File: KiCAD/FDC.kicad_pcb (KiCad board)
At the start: 2 copper layers, 72.6 x 65.5 mm, 26 parts, among them J2 Conn_02x20_Odd_Even, J3 SD_Card, Q1 SSM3K324RLFCT-ND, Q2 SSM3K324RLFCT-ND, U1 SN74LVCC4245ADWR, U2 Pico, U3 SN74LVCC4245ADWR, U4 SN74LVCC4245ADWR, U5 SN74LVCC4245ADWR

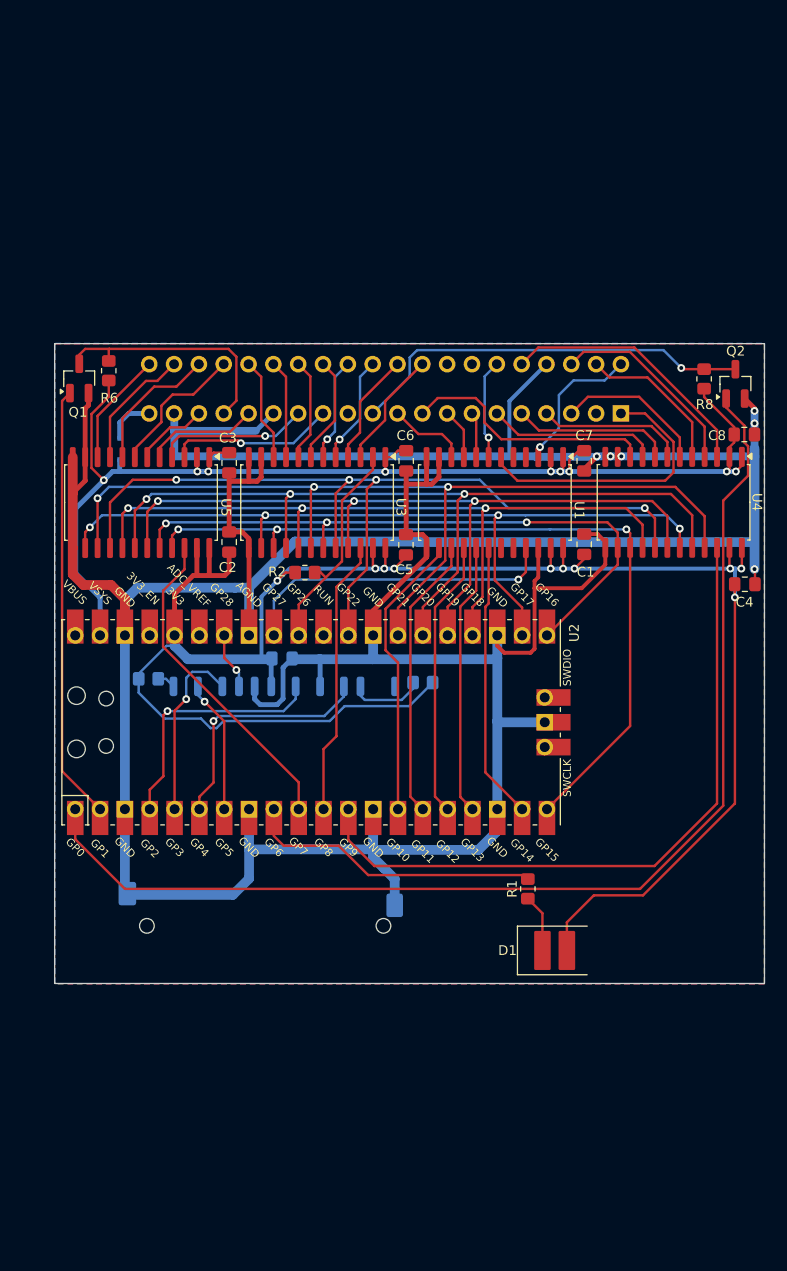
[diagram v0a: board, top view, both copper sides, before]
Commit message: First upload of test board.
First upload of test board.
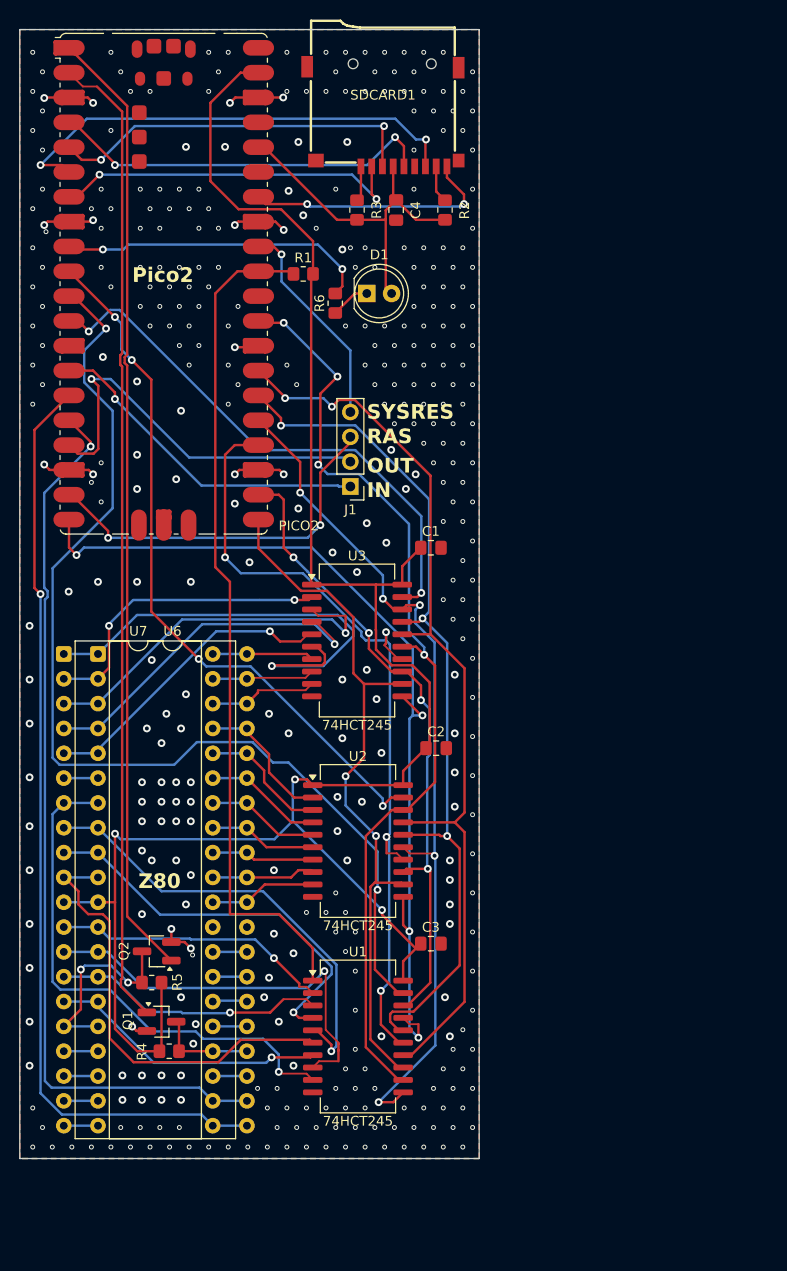
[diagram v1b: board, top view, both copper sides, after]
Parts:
- removed the C4 at (182.7, 80.7)
- removed C5, C6, C7, C8: 100nF, Capacitor_SMD:C_0805_2012Metric_Pad1.18x1.45mm_HandSolder
- removed D2: PMEG4010CEJ, Diode_SMD:D_SOD-323F
- removed J2: Conn_02x20_Odd_Even, Connector_PinSocket_2.54mm:PinSocket_2x20_P2.54mm_Vertical
- removed J3: SD_Card, Connector_Card:SD_Kyocera_145638009511859+
- removed the R2 at (137.7, 79.6)
- removed U4, U5: SN74LVCC4245ADWR, Package_SO:SOIC-24W_7.5x15.4mm_P1.27mm
- added J1: Conn_01x04, Connector_PinHeader_2.54mm:PinHeader_1x04_P2.54mm_Vertical, F.Cu at (142.3, 70.7)
- added R1: 1k, Resistor_SMD:R_0805_2012Metric_Pad1.20x1.40mm_HandSolder, F.Cu at (137.5, 49.0)
- added SDCARD1: ST-TF-003A, 00-ProjectLib:MicroSD_Card_TB, F.Cu at (145.7, 38.8)
- added U2: 74HCT245, Package_SO:SOIC-20W_7.5x15.4mm_P1.27mm, F.Cu at (143.1, 107.0)
- added U6: Z80, Package_DIP:DIP-40_W15.24mm, F.Cu at (116.5, 87.9)
- added U7: Z80, Package_DIP:DIP-40_W15.24mm, F.Cu at (113.0, 87.9)
- C4: renamed from C9; moved to F.Cu
- D1: footprint LED_SMD:LED_2816_7142Metric_Pad3.20x4.45mm_HandSolder -> LED_THT:LED_D5.0mm
- PICO2: renamed from U2; value Pico -> Pico 2; footprint MCU_RaspberryPi_and_Boards:RPi_Pico_SMD_TH -> Module:RaspberryPi_Pico_SMD
- Q1, Q2: value SSM3K324RLFCT-ND -> 2N7002
- R2: renamed from R3; moved to F.Cu
- R3: renamed from R4; moved to F.Cu
- U1, U3: value SN74LVCC4245ADWR -> 74HCT245; footprint Package_SO:SOIC-24W_7.5x15.4mm_P1.27mm -> Package_SO:SOIC-20W_7.5x15.4mm_P1.27mm
- moved R5 83.7 mm to (122.0, 121.5), turned to 0 degrees
- moved Q2 82.9 mm to (122.5, 118.3), turned to 180 degrees
- moved D1 69.9 mm to (144.0, 51.0)
- moved R4 69.9 mm to (123.8, 128.5), turned to 180 degrees
- moved Q1 66.3 mm to (123.0, 125.5), turned to 0 degrees
- moved R6 63.1 mm to (140.8, 52.0)
- moved U1 56.4 mm to (143.1, 127.0), turned to 0 degrees
- moved C3 53.3 mm to (150.6, 117.5), turned to 0 degrees
- moved R3 52.5 mm to (143.0, 42.5), turned to -90 degrees
- moved R2 48.4 mm to (152.0, 42.5), turned to 90 degrees
- moved C4 47.3 mm to (147.0, 42.5), turned to -90 degrees
- moved PICO2 47.3 mm to (123.2, 50.0), turned to 0 degrees
- moved C2 29.9 mm to (151.1, 97.5), turned to 0 degrees
- moved C1 15.7 mm to (150.6, 77.0), turned to 0 degrees
- moved U3 14.7 mm to (143.0, 86.5), turned to 0 degrees
- renumbered R6 to R4, R8 to R5, R1 to R6
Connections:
- C1 pad 1: +3V3 -> +5V
- C2 pad 1: +3V3 -> +5V
- PICO2 pad 15: /RD' -> /RD*
- PICO2 pad 16: /WR' -> /WR*
- R2 pad 1: Net-(J3-DAT1) -> +3V3
- R2 pad 2: +3V3 -> Net-(SDCARD1-DAT1)
- U1 pad 1: +5V -> /DIR
- U1 pad 10: /IN* -> GND
- U1 pad 11: GND -> /D4'
- U1 pad 12: GND -> /D7'
- U1 pad 13: GND -> /D1'
- U1 pad 14: /IN' -> /D6'
- U1 pad 15: /RD' -> /D3'
- U1 pad 16: /WR' -> /D5'
- U1 pad 17: /OUT' -> /D0'
- U1 pad 18: /MREQ' -> /D2'
- U1 pad 19: unconnected-(U1-B3-Pad19) -> /DATAB_OE
- U1 pad 2: +5V -> /D2
- U1 pad 20: unconnected-(U1-B2-Pad20) -> +5V
- U1 pad 3: /SYSRES* -> /D0
- U1 pad 4: unconnected-(U1-A2-Pad4) -> /D5
- U1 pad 5: unconnected-(U1-A3-Pad5) -> /D3
- U1 pad 6: /RAS* -> /D6
- U1 pad 7: /OUT* -> /D1
- U1 pad 8: /WR* -> /D7
- U1 pad 9: /RD* -> /D4
- U3 pad 10: /D2 -> GND
- U3 pad 11: GND -> /D0'
- U3 pad 12: GND -> /D1'
- U3 pad 13: GND -> /D2'
- U3 pad 14: /D2' -> /D3'
- U3 pad 15: /D0' -> /D7'
- U3 pad 16: /D5' -> /D6'
- U3 pad 17: /D3' -> /D5'
- U3 pad 18: /D6' -> /D4'
- U3 pad 19: /D1' -> /ADDRH_OE
- U3 pad 2: /DIR -> /A12
- U3 pad 20: /D7' -> +5V
- U3 pad 3: /D4 -> /A13
- U3 pad 4: /D7 -> /A14
- U3 pad 5: /D1 -> /A15
- U3 pad 6: /D6 -> /A11
- U3 pad 7: /D3 -> /A10
- U3 pad 8: /D5 -> /A9
- U3 pad 9: /D0 -> /A8
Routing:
- net GND: track 446.6 -> 40.2 mm, vias 6 -> 388
- net +3V3: track 199.1 -> 35.8 mm, vias 10 -> 0
- net /RD*: track 5.17 -> 96.1 mm, vias 0 -> 1
- net /WR*: track 4.64 -> 92.3 mm, vias 0 -> 1
- net /DATAB_OE: track 28.3 -> 109.0 mm, vias 0 -> 2
- net +5V: track 122.9 -> 197.1 mm, vias 9 -> 3
- net /DIR: track 22.7 -> 87.8 mm
- net /WAIT': track 44.5 -> 100.5 mm
- net /D4: track 12.1 -> 54.2 mm, vias 0 -> 1
- net /ADDRL_OE: track 33.4 -> 73.1 mm, vias 0 -> 4
- net /D6: track 10.6 -> 45.7 mm, vias 1 -> 0
- net /D3: track 11.0 -> 45.9 mm, vias 0 -> 1
- net /A11: track 16.4 -> 50.1 mm, vias 0 -> 1
- net /D5: track 10.5 -> 40.7 mm, vias 0 -> 1
- net /D7: track 11.6 -> 41.7 mm, vias 0 -> 1
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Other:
- board size 72.6 x 65.5 mm -> 47 x 115.5 mm
- board text added: "IN"
- board text added: "OUT"
- board text added: "Pico2"
- board text added: "Q1,Q2 - 2N7002 R1,R2,R3,R4,R5 - 1k C1,C2,C3,C4 - 100NF R6 - 100 OHM U1,U2,U3 - 74HCT245"
- board text added: "RAS"
- board text added: "SYSRES"
- board text added: "Z80"

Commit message: New PCB.. this may fit
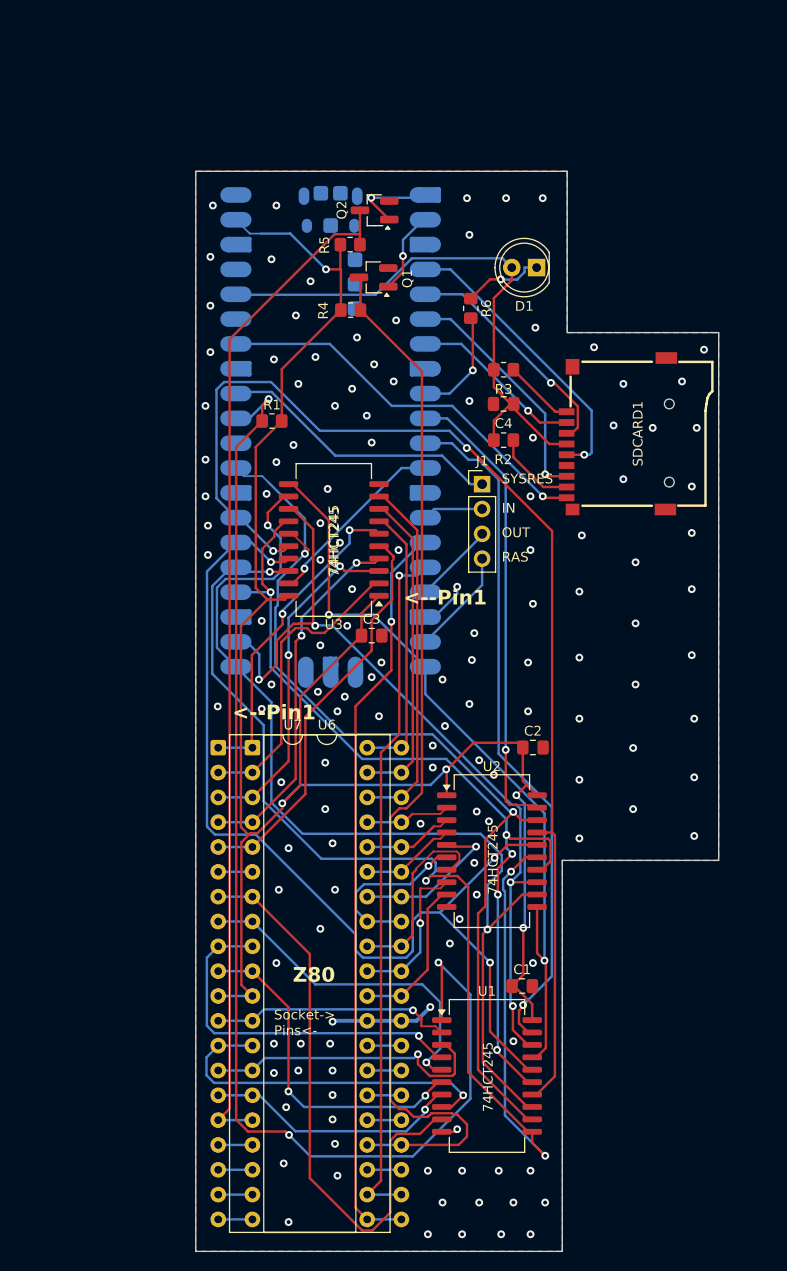
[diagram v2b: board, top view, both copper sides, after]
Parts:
- PICO2: moved to B.Cu
- moved Q1 79.2 mm to (144.7, 49.4), turned to 180 degrees
- moved Q2 79.0 mm to (144.8, 42.5)
- moved R5 78.2 mm to (142.3, 46.0), turned to 180 degrees
- moved R4 78.1 mm to (142.3, 52.7)
- moved SDCARD1 32.1 mm to (163.7, 65.3), turned to -90 degrees
- moved R2 24.3 mm to (158.0, 66.0), turned to 0 degrees
- moved PICO2 22.8 mm to (140.3, 65.0), turned to 180 degrees
- moved C4 22.7 mm to (158.0, 62.3), turned to 180 degrees
- moved R3 22.2 mm to (158.0, 58.8), turned to 180 degrees
- moved U6 18.5 mm to (132.3, 97.5)
- moved U7 18.5 mm to (128.8, 97.5)
- moved D1 17.6 mm to (161.4, 48.4), turned to 180 degrees
- moved R1 15.4 mm to (134.3, 64.0)
- moved R6 13.9 mm to (154.6, 52.5), turned to -90 degrees
- moved U1 13.8 mm to (156.3, 131.1)
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- renumbered C3 to C1, C1 to C3
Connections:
- J1 pad 1: /IN' -> /SYSRES'
- J1 pad 2: /OUT' -> /IN'
- J1 pad 3: /MREQ' -> /OUT'
- J1 pad 4: /SYSRES' -> /MREQ'
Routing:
- net /WAIT*: track 10.1 -> 109.6 mm
- net /WAIT': track 100.5 -> 8.54 mm, vias 0 -> 1
- net /INT': track 97.9 -> 8.64 mm, vias 0 -> 1
- net /INT*: track 20.4 -> 105.2 mm, vias 2 -> 0
- net /DIR: track 87.8 -> 128.6 mm, vias 0 -> 3
- net /DATAB_OE: track 109.0 -> 70.1 mm, vias 2 -> 1
- net /D4': track 88.8 -> 126.0 mm, vias 5 -> 4
- net /ADDRH_OE: track 56.1 -> 19.3 mm, vias 2 -> 1
- net /OUT': track 41.0 -> 8.38 mm, vias 1 -> 0
- net /D1': track 72.9 -> 102.2 mm
- net /IN': track 34.1 -> 6.18 mm, vias 1 -> 0
- net /MREQ': track 38.8 -> 10.9 mm, vias 2 -> 0
- net /D6': track 95.5 -> 122.4 mm
- net /ADDRL_OE: track 73.1 -> 47.4 mm, vias 4 -> 1
- net /A8: track 11.1 -> 36.8 mm
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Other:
- board size 47 x 115.5 mm -> 53.5 x 110.5 mm
- board text added: "74HCT245"
- board text added: "<--Pin1"
- board text added: "Floppy80-M1 Internal version by dabone 2026 https://github.com/dabonetn/Floppy80-M1-Internal"
- board text added: "Socket-> Pins<-"
- board text removed: "Pico2"
